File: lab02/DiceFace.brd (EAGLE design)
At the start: 160 x 100 mm, 1 part

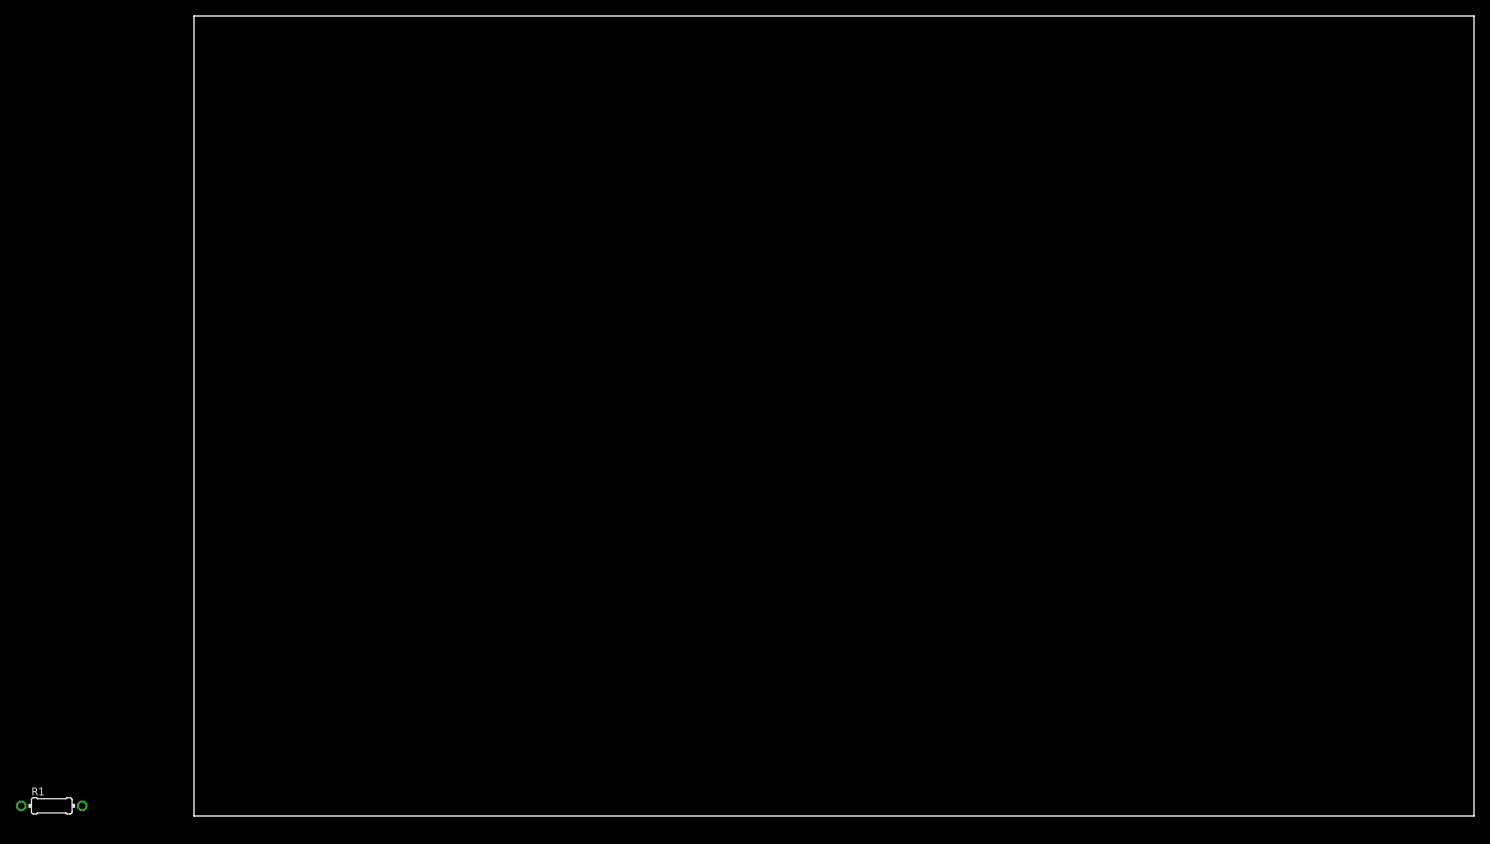
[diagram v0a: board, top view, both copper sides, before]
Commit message: Board shape and prod files
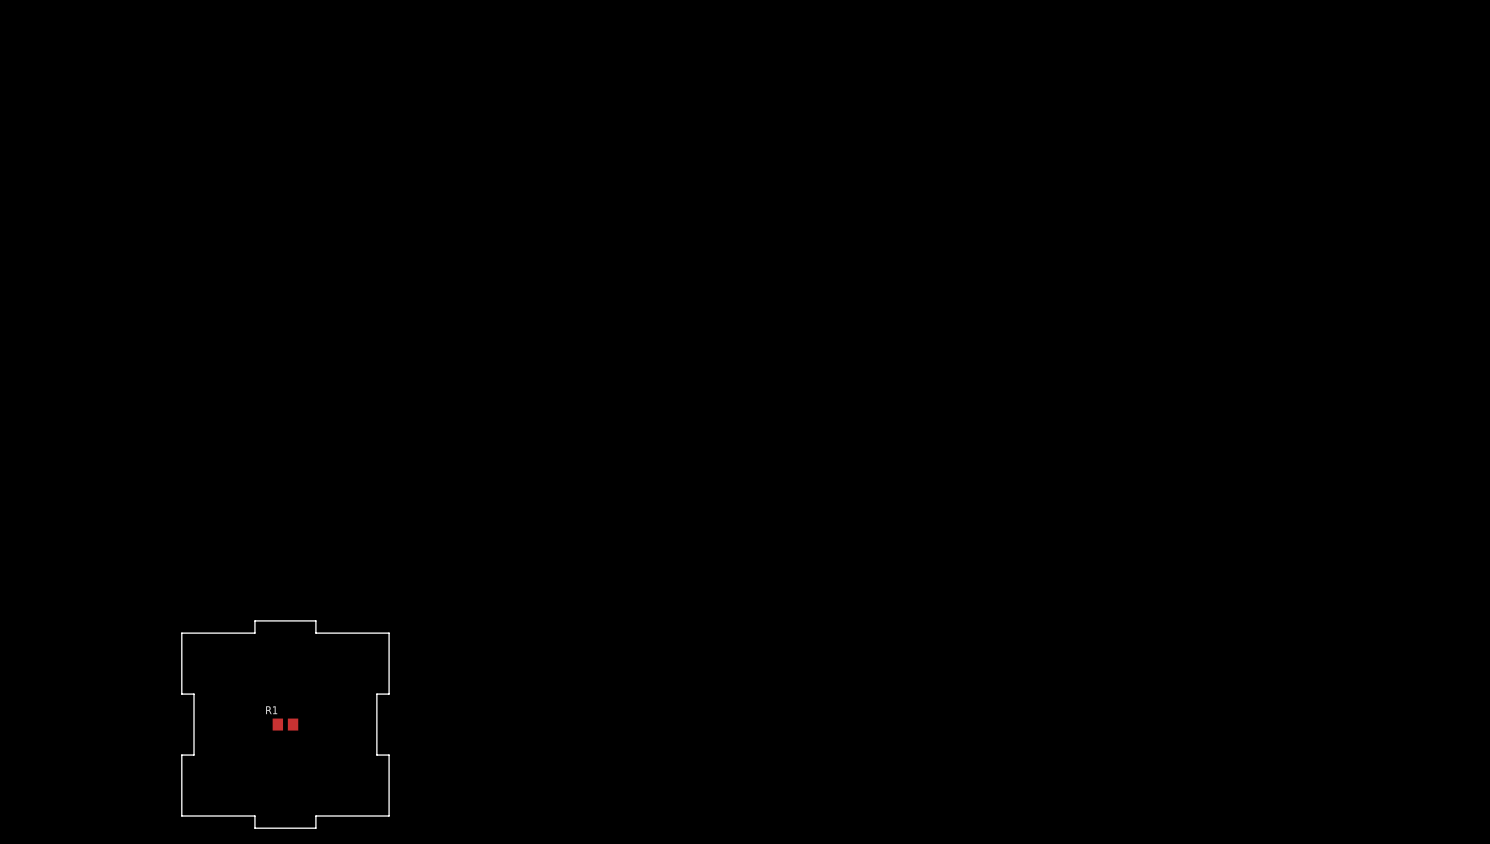
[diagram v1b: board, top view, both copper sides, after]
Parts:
- R1: device resistor:0204/7 -> resistor:R0805
- moved R1 30.9 mm to (11.4, 11.4)
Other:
- board size 160 x 100 mm -> 25.9 x 25.9 mm
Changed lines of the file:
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@@
 <drawing>
 <settings>
-<setting alwaysvectorfont="no"/>
+<setting alwaysvectorfont="yes"/>
 <setting verticaltext="up"/>
 </settings>
@@
 <layer number="98" name="Guide" color="6" fill="1" visible="no" active="no"/>
 <layer number="99" name="SpiceOrder" color="5" fill="1" visible="no" active="no"/>
+<layer number="200" name="200bmp" color="1" fill="10" visible="no" active="yes"/>
 </layers>
 <board>
 <plain>
-<wire x1="0" y1="0" x2="160" y2="0" width="0" layer="20"/>
-<wire x1="160" y1="0" x2="160" y2="100" width="0" layer="20"/>
-<wire x1="160" y1="100" x2="0" y2="100" width="0" layer="20"/>
-<wire x1="0" y1="100" x2="0" y2="0" width="0" layer="20"/>
+<wire x1="-1.524" y1="0" x2="7.62" y2="0" width="0" layer="20"/>
+<wire x1="7.62" y1="0" x2="7.62" y2="-1.524" width="0" layer="20"/>
+<wire x1="7.62" y1="-1.524" x2="15.24" y2="-1.524" width="0" layer="20"/>
+<wire x1="15.24" y1="-1.524" x2="15.24" y2="0" width="0" layer="20"/>
+<wire x1="15.24" y1="0" x2="24.384" y2="0" width="0" layer="20"/>
+<wire x1="24.384" y1="0" x2="24.384" y2="7.62" width="0" layer="20"/>
+<wire x1="24.384" y1="7.62" x2="22.86" y2="7.62" width="0" layer="20"/>
+<wire x1="22.86" y1="7.62" x2="22.86" y2="15.24" width="0" layer="20"/>
+<wire x1="22.86" y1="15.24" x2="24.384" y2="15.24" width="0" layer="20"/>
+<wire x1="24.384" y1="15.24" x2="24.384" y2="22.86" width="0" layer="20"/>
+<wire x1="24.384" y1="22.86" x2="15.24" y2="22.86" width="0" layer="20"/>
+<wire x1="15.24" y1="22.86" x2="15.24" y2="24.384" width="0" layer="20"/>
+<wire x1="15.24" y1="24.384" x2="7.62" y2="24.384" width="0" layer="20"/>
+<wire x1="7.62" y1="24.384" x2="7.62" y2="22.86" width="0" layer="20"/>
+<wire x1="7.62" y1="22.86" x2="-1.524" y2="22.86" width="0" layer="20"/>
+<wire x1="-1.524" y1="22.86" x2="-1.524" y2="15.24" width="0" layer="20"/>
+<wire x1="-1.524" y1="15.24" x2="0" y2="15.24" width="0" layer="20"/>
+<wire x1="0" y1="15.24" x2="0" y2="7.62" width="0" layer="20"/>
+<wire x1="0" y1="7.62" x2="-1.524" y2="7.62" width="0" layer="20"/>
+<wire x1="-1.524" y1="7.62" x2="-1.524" y2="0" width="0" layer="20"/>
 </plain>
 <attributes>
@@
 </autorouter>
 <elements>
-<element name="R1" library="resistor" library_urn="urn:adsk.eagle:library:348" package="0204/7" package3d_urn="urn:adsk.eagle:package:25945/1" value="" x="-17.78" y="1.27" smashed="yes">
-<attribute name="NAME" x="-20.32" y="2.5654" size="0.9906" layer="25" ratio="10"/>
-<attribute name="VALUE" x="-19.4056" y="0.7874" size="0.9906" layer="27" ratio="10"/>
+<element name="R1" library="resistor" library_urn="urn:adsk.eagle:library:348" package="R0805" package3d_urn="urn:adsk.eagle:package:26059/1" value="" x="11.43" y="11.43" smashed="yes">
+<attribute name="NAME" x="8.89" y="12.7254" size="0.9906" layer="25" ratio="10"/>
+<attribute name="VALUE" x="9.8044" y="10.9474" size="0.9906" layer="27" ratio="10"/>
 </element>
 </elements>
